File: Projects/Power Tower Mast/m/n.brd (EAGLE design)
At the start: 16.5 x 21.6 mm, 37 parts

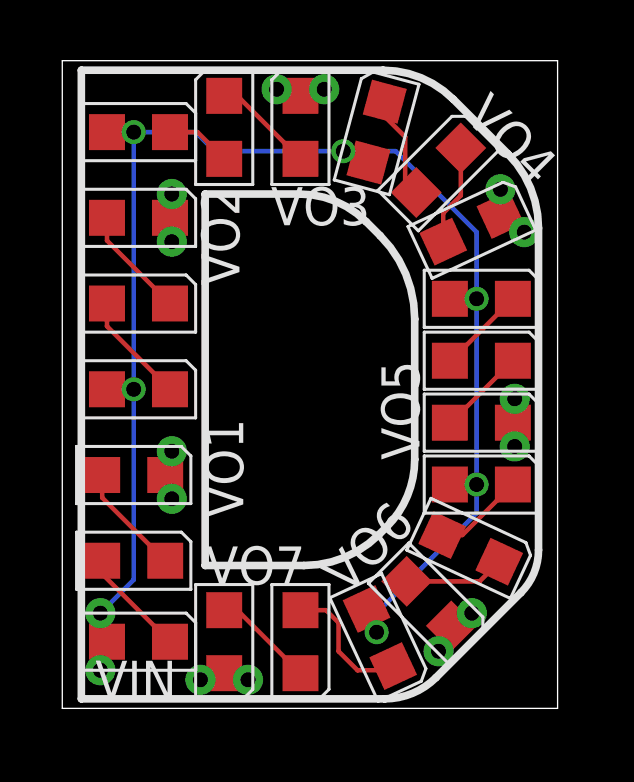
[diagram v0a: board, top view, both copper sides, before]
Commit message: final updates before fab.  added new letters for future projects.
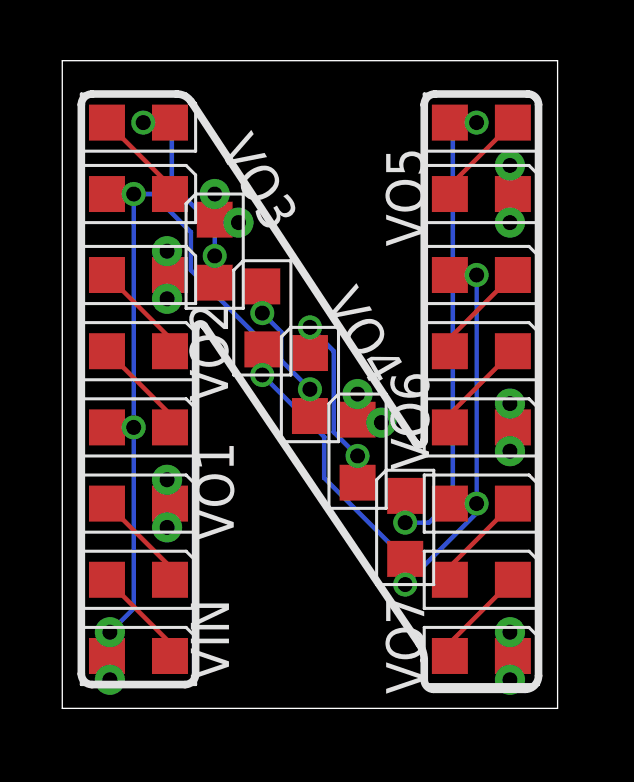
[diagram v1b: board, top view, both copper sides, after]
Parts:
- moved VO7 10.3 mm to (14.9, 0.95)
- moved VO14 8.87 mm to (14.9, 2.54)
- moved VO6 8.59 mm to (14.9, 10.2)
- moved LED21 8.59 mm to (14.0, 1.75), turned to 270 degrees
- moved LED12 8.35 mm to (9.84, 8.57), turned to 0 degrees
- moved LED11 8.33 mm to (8.26, 10.8), turned to 0 degrees
- moved VO11 8.32 mm to (9.84, 10.5)
- moved LED13 8.03 mm to (11.4, 6.03), turned to 0 degrees
- moved LED14 7.94 mm to (14.0, 19.5)
- moved VO4 7.94 mm to (10.6, 9.53)
- moved VO12 7.78 mm to (14.9, 18.1)
- moved LED15 7.62 mm to (14.0, 17.1)
- moved VO5 7.46 mm to (14.9, 16.2)
- moved LED10 7.27 mm to (6.67, 13.0), turned to 0 degrees
- moved LED16 6.98 mm to (14.0, 14.4)
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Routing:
- net N$48: track 2.95 -> 17.0 mm, vias 0 -> 2
- net N$43: track 3.41 -> 7.77 mm, vias 0 -> 2
- net N$45: track 3.37 -> 6.69 mm, vias 0 -> 2
- net VIN: track 51.8 -> 50.3 mm
- net N$46: track 3.46 -> 4.98 mm, vias 0 -> 2
- net N$1: track 4.54 -> 3.41 mm
- net N$44: track 2.18 -> 3.25 mm
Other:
- board text added: "N"
- board text removed: "D"
